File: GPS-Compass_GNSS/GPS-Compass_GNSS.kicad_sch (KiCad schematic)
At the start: 35 parts, among them J1 SMA_F, J3 01x10, Q1 MMBT3904, SW1 GNSS_RST, U1 BGA725L6E6327FTSA1, U2 TESEO-LIV3R

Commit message: asdas
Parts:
- J1: Antenna (none) -> https://cz.mouser.com/ProductDetail/Quectel/YEGT001AA?qs=7D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

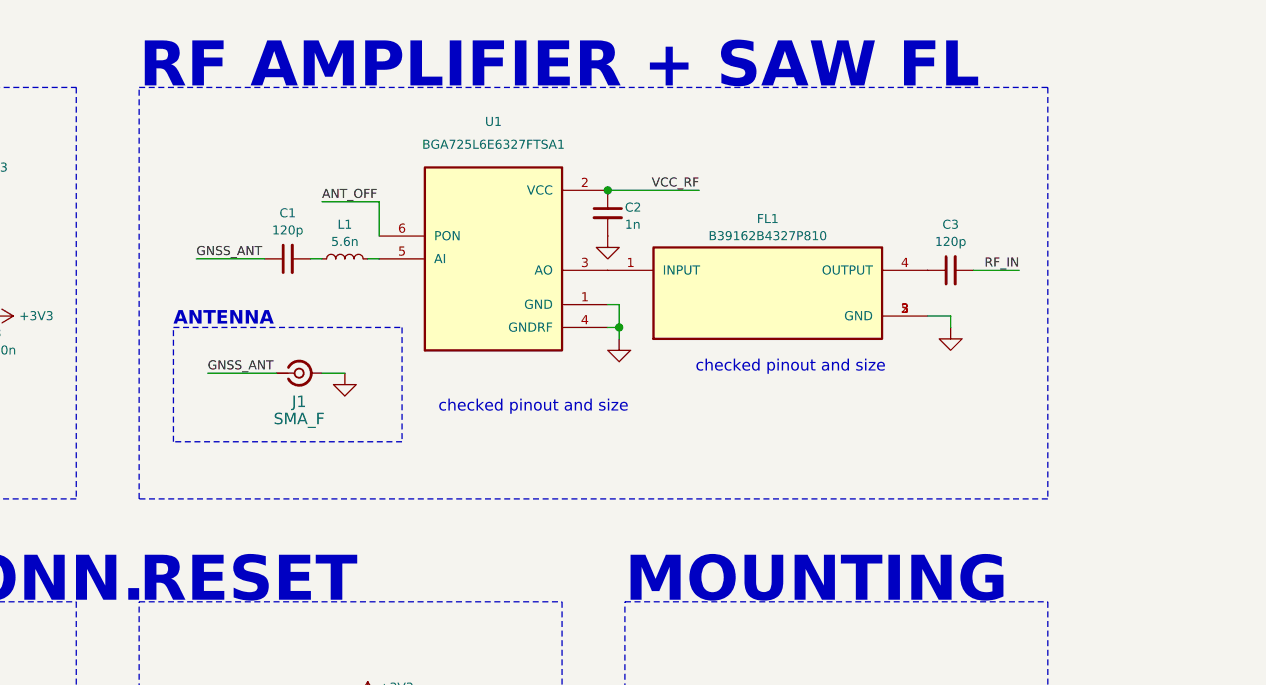
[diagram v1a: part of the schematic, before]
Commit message: updates on different boards
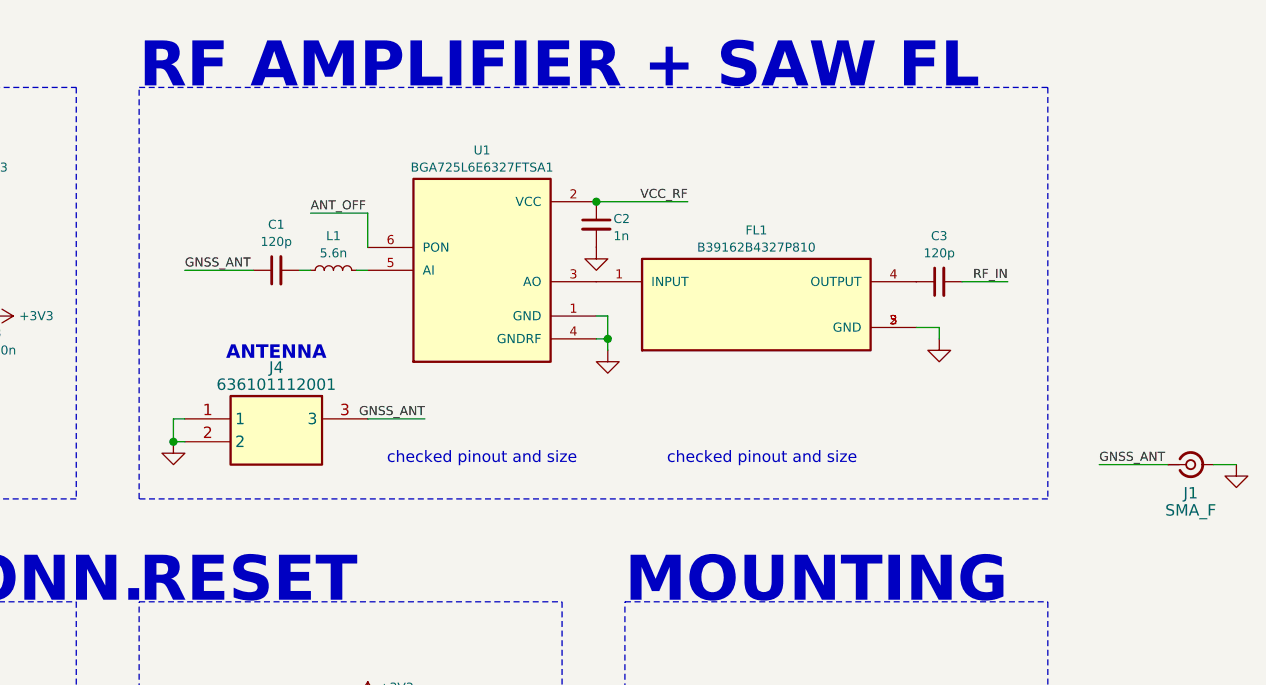
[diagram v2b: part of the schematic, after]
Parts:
- added J4: 636101112001, gps-compass_brd:636101112001, symbol gps-compass_sch:636101112001
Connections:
- net GND: now also J4.1, J4.2
- net GNSS_ANT: now also J4.3
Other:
- moved on the sheet: C1, C2, C3, FL1, J1, L1, U1
